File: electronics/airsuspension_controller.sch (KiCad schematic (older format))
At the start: 1 part

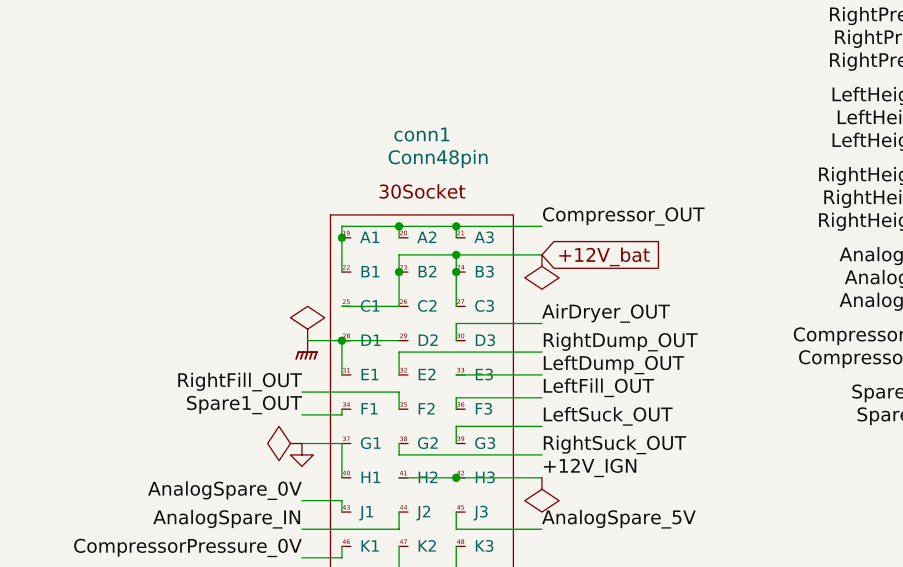
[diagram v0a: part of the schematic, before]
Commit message: PCB routing done
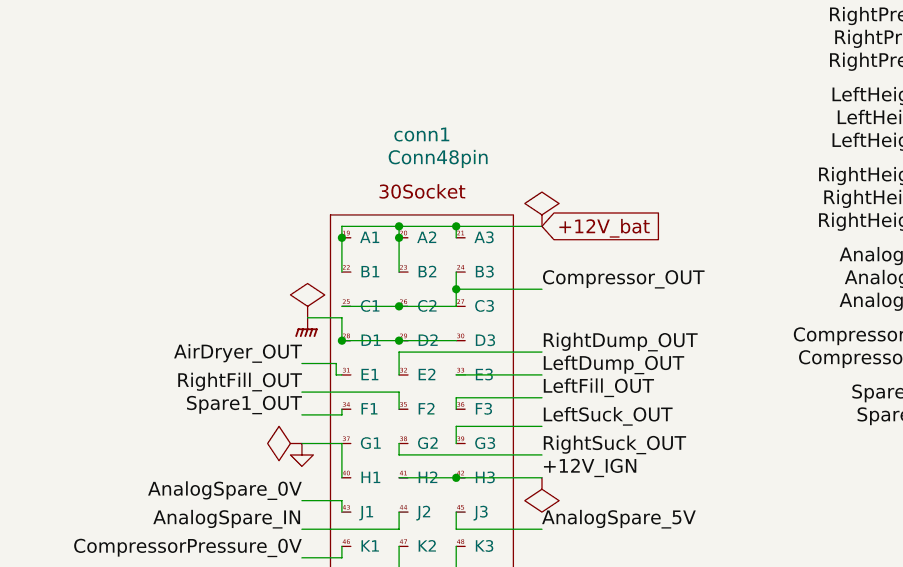
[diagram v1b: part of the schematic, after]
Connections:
- net +12V_bat: now also conn1.19 (A1), conn1.20 (A2), conn1.21 (A3), conn1.22 (B1); no longer conn1.24 (B3), conn1.25 (C1), conn1.26 (C2), conn1.27 (C3)
- net AirDryer_OUT: now also conn1.31 (E1); no longer conn1.30 (D3)
- net Compressor_OUT: now also conn1.24 (B3), conn1.25 (C1), conn1.26 (C2), conn1.27 (C3); no longer conn1.19 (A1), conn1.20 (A2), conn1.21 (A3), conn1.22 (B1)
- net GNDPWR: now also conn1.30 (D3); no longer conn1.31 (E1)
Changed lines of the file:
@@
 Text Label 9650 5150 2    60   ~ 0
 CAN_RX
-Text Label 2825 2275 0    60   ~ 0
+Text Label 2825 2550 0    60   ~ 0
 Compressor_OUT
-Text GLabel 2825 2400 2    60   Input ~ 0
+Text GLabel 2825 2275 2    60   Input ~ 0
 +12V_bat
 $Comp
 L PWR_FLAG #FLG01
 U 1 1 56FCC0F2
-P 2825 2400
-F 0 "#FLG01" H 2825 2495 50  0001 C CNN
-F 1 "PWR_FLAG" H 2825 2624 50  0001 C CNN
-F 2 "" H 2825 2400 50  0000 C CNN
-F 3 "" H 2825 2400 50  0000 C CNN
-	1    2825 2400
-	-1   0    0    1
+P 2825 2275
+F 0 "#FLG01" H 2825 2370 50  0001 C CNN
+F 1 "PWR_FLAG" H 2825 2499 50  0001 C CNN
+F 2 "" H 2825 2275 50  0000 C CNN
+F 3 "" H 2825 2275 50  0000 C CNN
+	1    2825 2275
+	1    0    0    -1
 $EndComp
 $Comp
 L PWR_FLAG #FLG02
 U 1 1 56FCC0F8
-P 1800 2775
-F 0 "#FLG02" H 1800 2870 50  0001 C CNN
-F 1 "PWR_FLAG" H 1800 2999 50  0001 C CNN
-F 2 "" H 1800 2775 50  0000 C CNN
-F 3 "" H 1800 2775 50  0000 C CNN
-	1    1800 2775
+P 1800 2675
+F 0 "#FLG02" H 1800 2770 50  0001 C CNN
+F 1 "PWR_FLAG" H 1800 2899 50  0001 C CNN
+F 2 "" H 1800 2675 50  0000 C CNN
+F 3 "" H 1800 2675 50  0000 C CNN
+	1    1800 2675
 	1    0    0    -1
 $EndComp
@@
 L GNDPWR #PWR03
 U 1 1 56FCC0FE
-P 1800 2775
-F 0 "#PWR03" H 1800 2575 50  0001 C CNN
-F 1 "GNDPWR" H 1807 2849 50  0001 C CNN
-F 2 "" H 1800 2725 50  0000 C CNN
-F 3 "" H 1800 2725 50  0000 C CNN
-	1    1800 2775
+P 1800 2675
+F 0 "#PWR03" H 1800 2475 50  0001 C CNN
+F 1 "GNDPWR" H 1807 2749 50  0001 C CNN
+F 2 "" H 1800 2625 50  0000 C CNN
+F 3 "" H 1800 2625 50  0000 C CNN
+	1    1800 2675
 	1    0    0    -1
 $EndComp
@@
 Text Label 2825 3150 0    60   ~ 0
 LeftSuck_OUT
-Text Label 2825 2700 0    60   ~ 0
+Text Label 1775 2875 2    60   ~ 0
 AirDryer_OUT
 Text Label 1775 3100 2    60   ~ 0
@@
 	-1   0    0    1
 $EndComp
-Wire Wire Line
-	2200 3225 2200 3275
-Wire Wire Line
-	2200 3275 2825 3275
-Wire Wire Line
-	2450 3225 2450 3150
-Wire Wire Line
-	2450 3150 2825 3150
-Wire Wire Line
-	2200 3375 2825 3375
-Wire Wire Line
-	2200 5075 2200 5250
-Wire Wire Line
-	2200 5250 2825 5250
-Wire Wire Line
-	2450 5075 2450 5125
-Wire Wire Line
-	2450 5125 2825 5125
-Wire Wire Line
-	1950 5075 1950 5125
-Wire Wire Line
-	1950 5125 1775 5125
-Wire Wire Line
-	1950 4925 1950 4900
-Wire Wire Line
-	1950 4900 1775 4900
-Wire Wire Line
-	2200 4775 2200 4825
-Wire Wire Line
-	2200 4825 2825 4825
-Wire Wire Line
-	2450 4775 2450 4725
-Wire Wire Line
-	2450 4725 2825 4725
-Wire Wire Line
-	1950 4775 1775 4775
-Wire Wire Line
-	2200 4625 2200 4675
-Wire Wire Line
-	2200 4675 1775 4675
-Wire Wire Line
-	1950 4625 1950 4575
-Wire Wire Line
-	1950 4575 1775 4575
-Wire Wire Line
-	2450 4625 2825 4625
-Wire Wire Line
-	2200 4475 2200 4525
-Wire Wire Line
-	2200 4525 2825 4525
-Wire Wire Line
-	2450 4475 2450 4425
-Wire Wire Line
-	2450 4425 2825 4425
-Wire Wire Line
-	1950 4475 1775 4475
-Wire Wire Line
-	2200 4325 2200 4375
-Wire Wire Line
-	2200 4375 1775 4375
-Wire Wire Line
-	1950 4325 1950 4275
-Wire Wire Line
-	1950 4275 1775 4275
-Wire Wire Line
-	2450 4325 2825 4325
-Wire Wire Line
-	1800 2775 2200 2775
-Wire Wire Line
-	2200 3075 2200 3000
-Connection ~ 1950 2325
-Wire Wire Line
-	2200 2400 2200 2625
-Wire Wire Line
-	2450 2400 2450 2625
-Wire Wire Line
-	2200 2400 2825 2400
-Connection ~ 2200 2475
-Connection ~ 2450 2400
-Connection ~ 2450 2475
-Wire Wire Line
-	2200 2625 1950 2625
-Wire Wire Line
-	1950 2775 1950 2925
-Connection ~ 1950 2775
-Wire Wire Line
-	2450 2775 2450 2700
-Wire Wire Line
-	2450 2700 2825 2700
-Wire Wire Line
-	2200 2925 2200 2825
-Wire Wire Line
-	2200 2825 2825 2825
-Wire Wire Line
-	2450 2925 2825 2925
-Wire Wire Line
-	2200 3000 1775 3000
-Wire Wire Line
-	2450 3075 2450 3025
-Wire Wire Line
-	2450 3025 2825 3025
-Wire Wire Line
-	1950 3075 1950 3100
-Wire Wire Line
-	1950 3100 1775 3100
-Wire Wire Line
-	1950 3225 1950 3375
-Wire Wire Line
-	1950 3225 1775 3225
-Connection ~ 2450 3375
-Wire Wire Line
-	1950 3525 1950 3475
-Wire Wire Line
-	1950 3475 1775 3475
-Wire Wire Line
-	2200 3525 2200 3600
-Wire Wire Line
-	2200 3600 1775 3600
-Wire Wire Line
-	1950 3675 1950 3725
-Wire Wire Line
-	1950 3725 1775 3725
-Wire Wire Line
-	2200 3675 2200 3850
-Wire Wire Line
-	2200 3850 1775 3850
-Wire Wire Line
-	2450 3675 2450 3850
-Wire Wire Line
-	2450 3850 2825 3850
-Wire Wire Line
-	2450 3525 2450 3600
-Wire Wire Line
-	2450 3600 2825 3600
 $Comp
 L Conn48pin conn1
@@
 	1    0    0    -1
 $EndComp
-Wire Wire Line
-	2200 2275 2200 2325
-Wire Wire Line
-	2450 2275 2450 2325
-Wire Wire Line
-	1950 2275 1950 2475
-Wire Wire Line
-	1950 2275 2825 2275
-Connection ~ 2200 2275
-Connection ~ 2450 2275
-Wire Wire Line
-	2200 4925 2200 5000
-Wire Wire Line
-	2200 5000 1775 5000
-Wire Wire Line
-	2450 4925 2450 4975
-Wire Wire Line
-	2450 4975 2825 4975
 Text Label 4800 2800 2    60   ~ 0
 CompressorTemp_5V
 Text Label 4800 2900 2    60   ~ 0
 CompressorTemp_IN
+Wire Wire Line
+	2200 3225 2200 3275
+Wire Wire Line
+	2200 3275 2825 3275
+Wire Wire Line
+	2450 3225 2450 3150
+Wire Wire Line
+	2450 3150 2825 3150
+Wire Wire Line
+	2200 3375 2825 3375
+Wire Wire Line
+	2200 5075 2200 5250
+Wire Wire Line
+	2200 5250 2825 5250
+Wire Wire Line
+	2450 5075 2450 5125
+Wire Wire Line
+	2450 5125 2825 5125
+Wire Wire Line
+	1950 5075 1950 5125
+Wire Wire Line
+	1950 5125 1775 5125
+Wire Wire Line
+	1950 4925 1950 4900
+Wire Wire Line
+	1950 4900 1775 4900
+Wire Wire Line
+	2200 4775 2200 4825
+Wire Wire Line
+	2200 4825 2825 4825
+Wire Wire Line
+	2450 4775 2450 4725
+Wire Wire Line
+	2450 4725 2825 4725
+Wire Wire Line
+	1950 4775 1775 4775
+Wire Wire Line
+	2200 4625 2200 4675
+Wire Wire Line
+	2200 4675 1775 4675
+Wire Wire Line
+	1950 4625 1950 4575
+Wire Wire Line
+	1950 4575 1775 4575
+Wire Wire Line
+	2450 4625 2825 4625
+Wire Wire Line
+	2200 4475 2200 4525
+Wire Wire Line
+	2200 4525 2825 4525
+Wire Wire Line
+	2450 4475 2450 4425
+Wire Wire Line
+	2450 4425 2825 4425
+Wire Wire Line
+	1950 4475 1775 4475
+Wire Wire Line
+	2200 4325 2200 4375
+Wire Wire Line
+	2200 4375 1775 4375
+Wire Wire Line
+	1950 4325 1950 4275
+Wire Wire Line
+	1950 4275 1775 4275
+Wire Wire Line
+	2450 4325 2825 4325
+Wire Wire Line
+	2200 3075 2200 3000
+Connection ~ 1950 2325
+Wire Wire Line
+	2450 2625 1950 2625
+Connection ~ 1950 2775
+Wire Wire Line
+	2200 2925 2200 2825
+Wire Wire Line
+	2200 2825 2825 2825
+Wire Wire Line
+	2450 2925 2825 2925
+Wire Wire Line
+	2200 3000 1775 3000
+Wire Wire Line
+	2450 3075 2450 3025
+Wire Wire Line
+	2450 3025 2825 3025
+Wire Wire Line
+	1950 3075 1950 3100
+Wire Wire Line
+	1950 3100 1775 3100
+Wire Wire Line
+	1950 3225 1950 3375
+Wire Wire Line
+	1950 3225 1775 3225
+Connection ~ 2450 3375
+Wire Wire Line
+	1950 3525 1950 3475
+Wire Wire Line
+	1950 3475 1775 3475
+Wire Wire Line
+	2200 3525 2200 3600
+Wire Wire Line
+	2200 3600 1775 3600
+Wire Wire Line
+	1950 3675 1950 3725
+Wire Wire Line
+	1950 3725 1775 3725
+Wire Wire Line
+	2200 3675 2200 3850
+Wire Wire Line
+	2200 3850 1775 3850
+Wire Wire Line
+	2450 3675 2450 3850
+Wire Wire Line
+	2450 3850 2825 3850
+Wire Wire Line
+	2450 3525 2450 3600
+Wire Wire Line
+	2450 3600 2825 3600
+Wire Wire Line
+	2200 2275 2200 2475
+Wire Wire Line
+	2450 2275 2450 2325
+Wire Wire Line
+	1950 2275 1950 2475
+Wire Wire Line
+	1950 2275 2825 2275
+Connection ~ 2200 2275
+Connection ~ 2450 2275
+Wire Wire Line
+	2200 4925 2200 5000
+Wire Wire Line
+	2200 5000 1775 5000
+Wire Wire Line
+	2450 4925 2450 4975
+Wire Wire Line
+	2450 4975 2825 4975
+Connection ~ 2200 2625
+Wire Wire Line
+	2450 2475 2450 2625
+Wire Wire Line
+	2825 2550 2450 2550
+Connection ~ 2450 2550
+Connection ~ 2200 2325
+Connection ~ 2200 2775
+Wire Wire Line
+	1950 2925 1925 2925
+Wire Wire Line
+	1950 2775 1950 2675
+Wire Wire Line
+	1950 2675 1800 2675
+Wire Wire Line
+	1950 2775 2450 2775
+Wire Wire Line
+	1925 2925 1925 2875
+Wire Wire Line
+	1925 2875 1775 2875
 $EndSCHEMATC
